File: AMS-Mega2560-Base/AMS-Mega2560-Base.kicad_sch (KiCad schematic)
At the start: 28 parts, among them IC6 OPA2340PA, J1 RTD1, J2 RTD2, J3 Conn_01x08, J31 Conn_01x02, J32 Conn_01x02, J4 Sense1, J5 Sense2, J6 AdafruitUltimateGPS, J7 Conn_02x03_Odd_Even, P1 Power, P10 CONN_01X01, P11 CONN_01X01, P12 CONN_01X01, P13 CONN_01X01, P2 Analog, P3 Analog, P4 Digital, P5 PWM, P6 PWM, P7 Communication, P8 CONN_01X01, P9 CONN_01X01

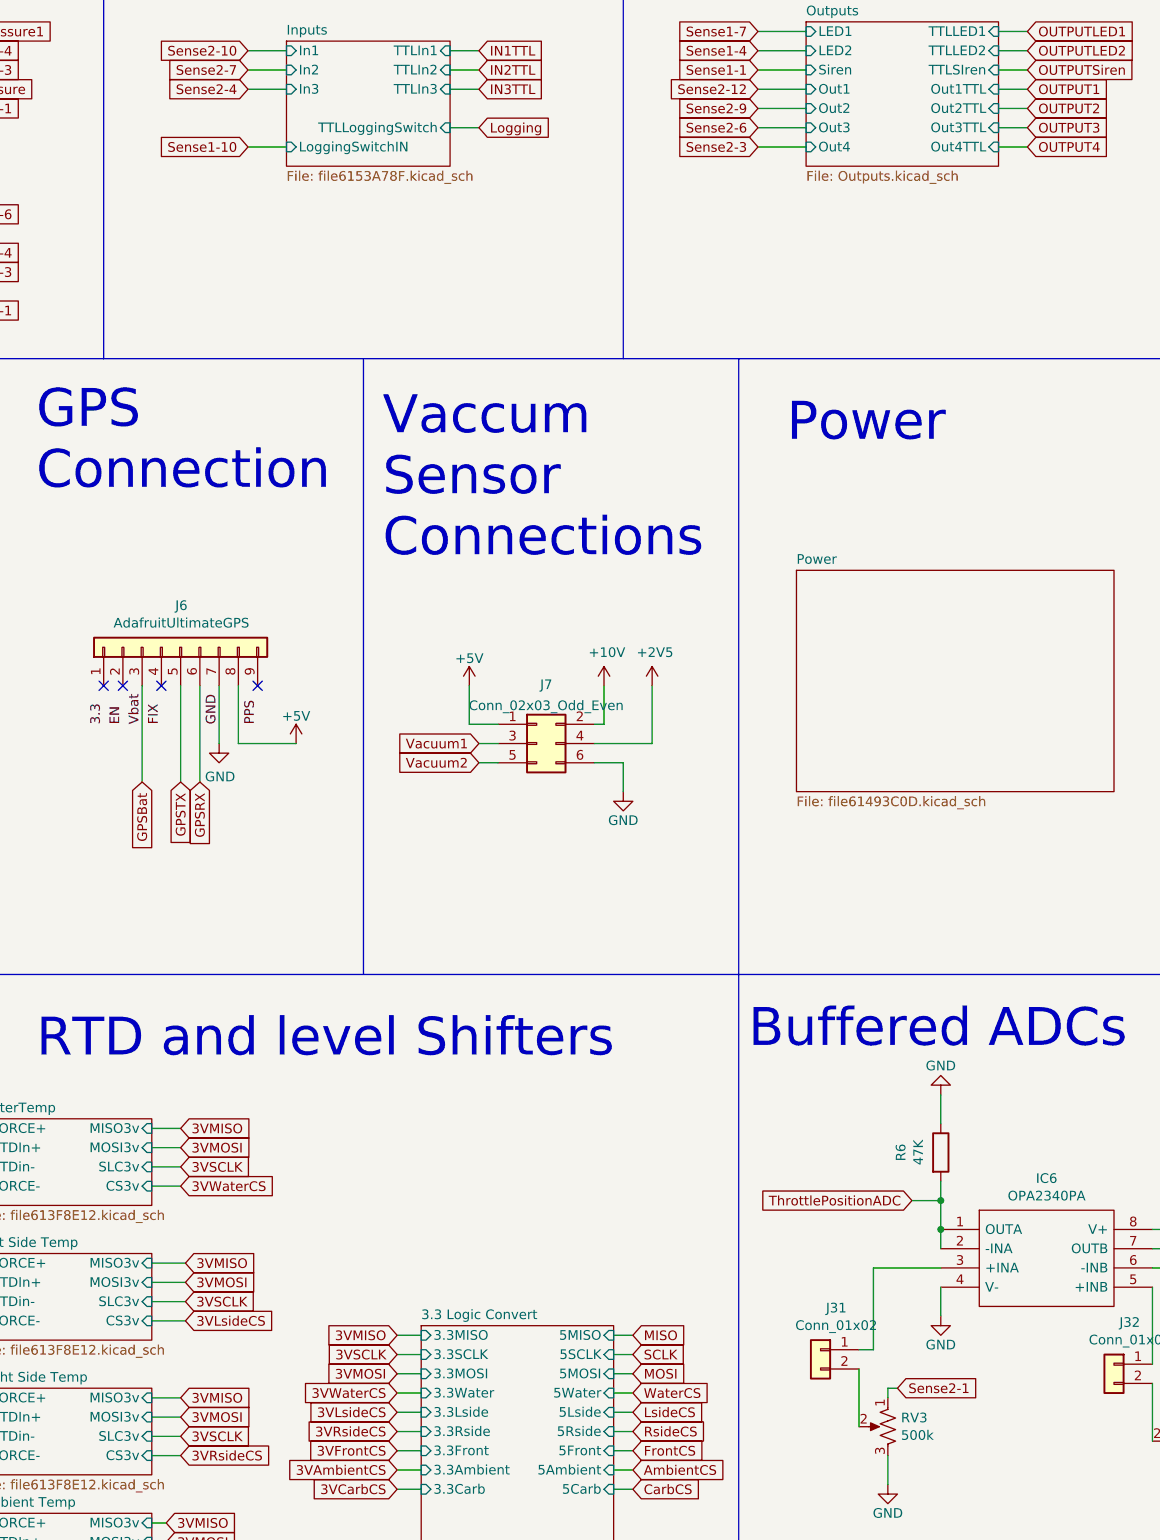
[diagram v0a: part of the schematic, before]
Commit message: pushing this change to the repo need to vet some schematics
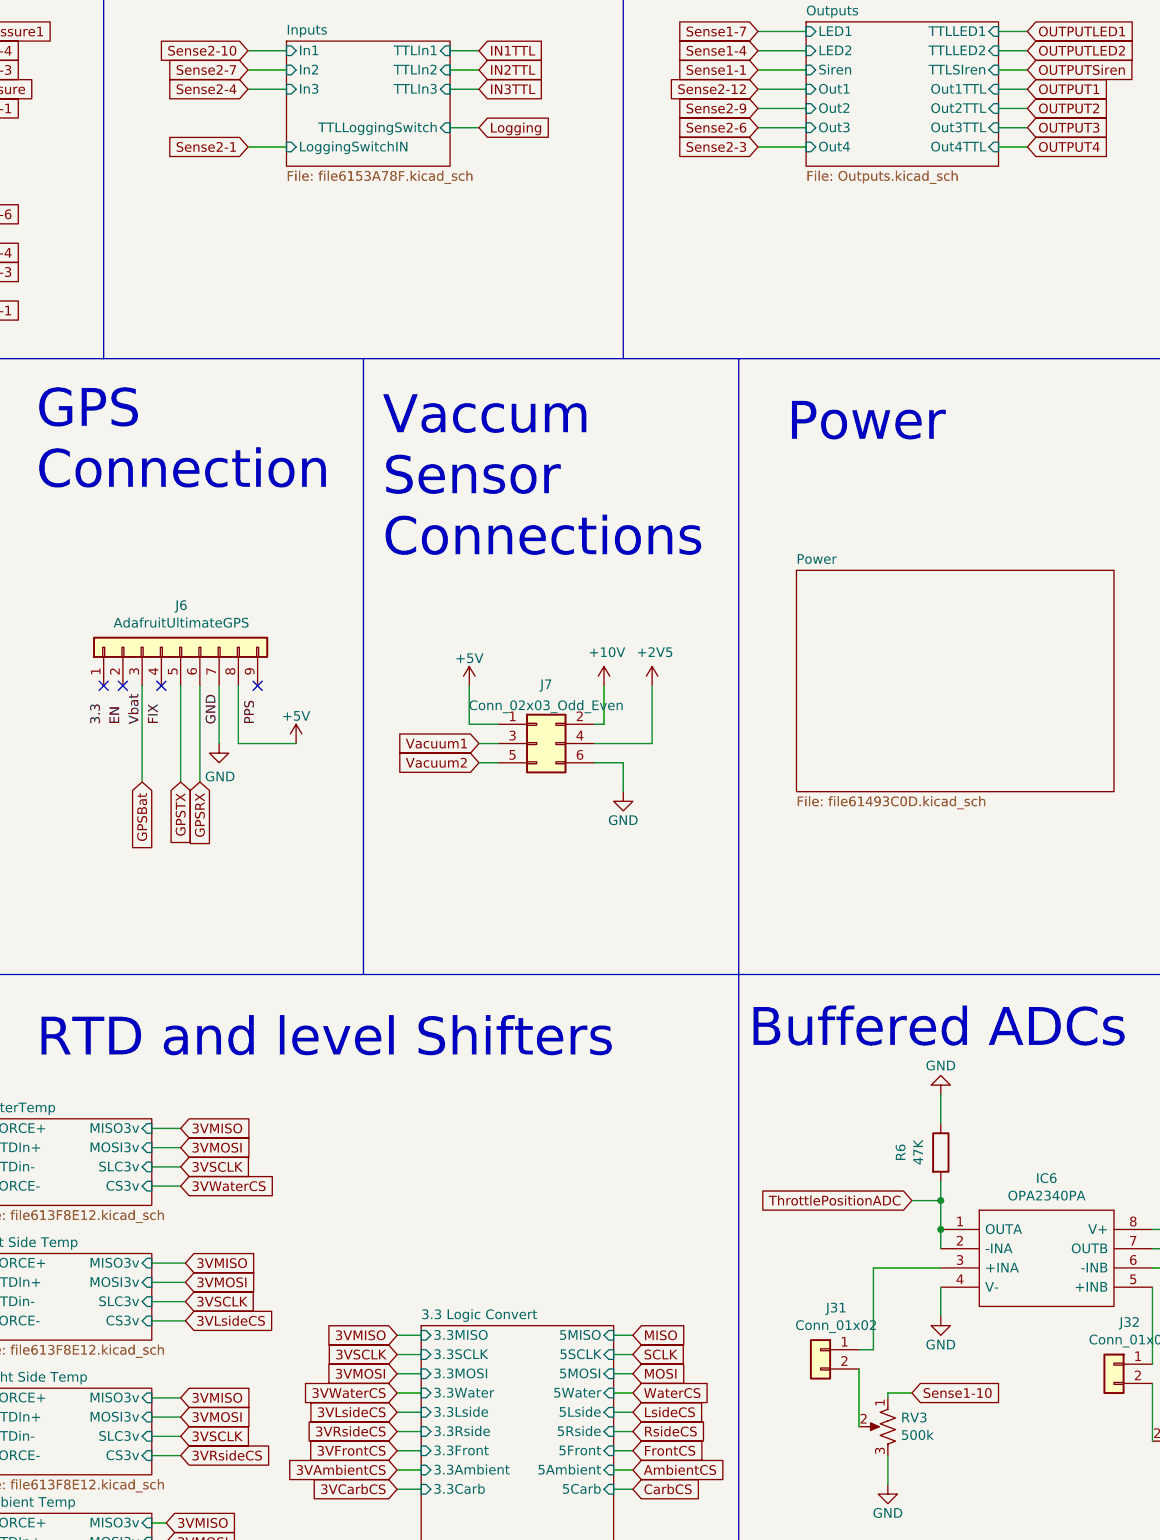
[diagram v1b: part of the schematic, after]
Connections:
- net Sense1-10: now also RV3.1
- net Sense2-1: no longer RV3.1
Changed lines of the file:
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@@
     (stroke (width 0) (type default) (color 0 0 0 0))
   )
-  (wire (pts (xy 177.8 207.01) (xy 177.8 196.215))
+  (wire (pts (xy 182.88 212.725) (xy 179.705 212.725))
     (stroke (width 0) (type default) (color 0 0 0 0))
   )
-  (wire (pts (xy 95.25 48.26) (xy 100.33 48.26))
+  (wire (pts (xy 177.8 207.01) (xy 177.8 196.215))
     (stroke (width 0) (type default) (color 0 0 0 0))
   )
@@
     (stroke (width 0) (type default) (color 0 0 0 0))
   )
-  (wire (pts (xy 179.705 213.36) (xy 179.705 212.09))
-    (stroke (width 0) (type default) (color 0 0 0 0))
-  )
   (wire (pts (xy 148.59 127) (xy 140.97 127))
     (stroke (width 0) (type default) (color 0 0 0 0))
@@
     (stroke (width 0) (type default) (color 0 0 0 0))
   )
-  (wire (pts (xy 179.705 212.09) (xy 180.975 212.09))
-    (stroke (width 0) (type default) (color 0 0 0 0))
-  )
   (wire (pts (xy 128.27 124.46) (xy 124.46 124.46))
     (stroke (width 0) (type default) (color 0 0 0 0))
@@
     (stroke (width 0) (type default) (color 0 0 0 0))
   )
+  (wire (pts (xy 179.705 212.725) (xy 179.705 213.36))
+    (stroke (width 0) (type default) (color 0 0 0 0))
+  )
   (wire (pts (xy 82.55 200.66) (xy 86.995 200.66))
     (stroke (width 0) (type default) (color 0 0 0 0))
@@
     (stroke (width 0) (type default) (color 0 0 0 0))
   )
+  (wire (pts (xy 95.25 48.26) (xy 100.33 48.26))
+    (stroke (width 0) (type default) (color 0 0 0 0))
+  )
   (wire (pts (xy 49.53 198.12) (xy 33.02 198.12))
     (stroke (width 0) (type default) (color 0 0 0 0))
@@
     )
   )
-  (global_label "Sense1-10" (shape input) (at 95.25 48.26 180) (fields_autoplaced)
-    (effects (font (size 1.27 1.27)) (justify right))
-    (property "Intersheet References" "${INTERSHEET_REFS}" (id 0) (at 82.161 48.1806 0)
-      (effects (font (size 1.27 1.27)) (justify right) hide)
+  (global_label "Sense1-10" (shape input) (at 182.88 212.725 0) (fields_autoplaced)
+    (effects (font (size 1.27 1.27)) (justify left))
+    (property "Intersheet References" "${INTERSHEET_REFS}" (id 0) (at 195.969 212.6456 0)
+      (effects (font (size 1.27 1.27)) (justify left) hide)
     )
   )
@@
     )
   )
-  (global_label "Sense2-1" (shape input) (at 180.975 212.09 0) (fields_autoplaced)
-    (effects (font (size 1.27 1.27)) (justify left))
-    (property "Intersheet References" "${INTERSHEET_REFS}" (id 0) (at 192.8544 212.0106 0)
-      (effects (font (size 1.27 1.27)) (justify left) hide)
+  (global_label "Sense2-1" (shape input) (at 95.25 48.26 180) (fields_autoplaced)
+    (effects (font (size 1.27 1.27)) (justify right))
+    (property "Intersheet References" "${INTERSHEET_REFS}" (id 0) (at 83.3706 48.1806 0)
+      (effects (font (size 1.27 1.27)) (justify right) hide)
     )
   )
@@
       (reference "Q21") (unit 1) (value "IRF9Z34NPBF") (footprint "SamacSys_Parts:TO254P469X1042X1967-3P")
     )
-    (path "/00000000-0000-0000-0000-000061493c0e/14fa351f-a44c-4cb9-86de-bc4ce1266c39"
-      (reference "Q22") (unit 1) (value "BD140") (footprint "Package_TO_SOT_THT:TO-126-3_Vertical")
+    (path "/00000000-0000-0000-0000-000061493c0e/54b9aef8-b50a-46a4-bd39-fa76fe97d610"
+      (reference "Q22") (unit 1) (value "IRF9610PBF-BE3") (footprint "TO254P465X1024X2050-3P")
     )
     (path "/00000000-0000-0000-0000-000061493c0e/26286b82-8e1d-44de-8c30-eae394d0f76a"
@@
       (reference "R63") (unit 1) (value "1M") (footprint "Resistor_THT:R_Axial_DIN0207_L6.3mm_D2.5mm_P2.54mm_Vertical")
     )
-    (path "/00000000-0000-0000-0000-00006152913d/98dbeacd-eda1-4446-87dd-ddc62165f2c4"
-      (reference "R64") (unit 1) (value "4.7K") (footprint "Resistor_THT:R_Axial_DIN0207_L6.3mm_D2.5mm_P2.54mm_Vertical")
-    )
     (path "/00000000-0000-0000-0000-0000614ca8f3/00000000-0000-0000-0000-0000614e2c3c"
